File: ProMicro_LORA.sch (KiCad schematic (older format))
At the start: 44 parts, among them J1 SMA, J2 COAX, U1 SX1276, U2 AS179-92LF, Y1 32Mhz

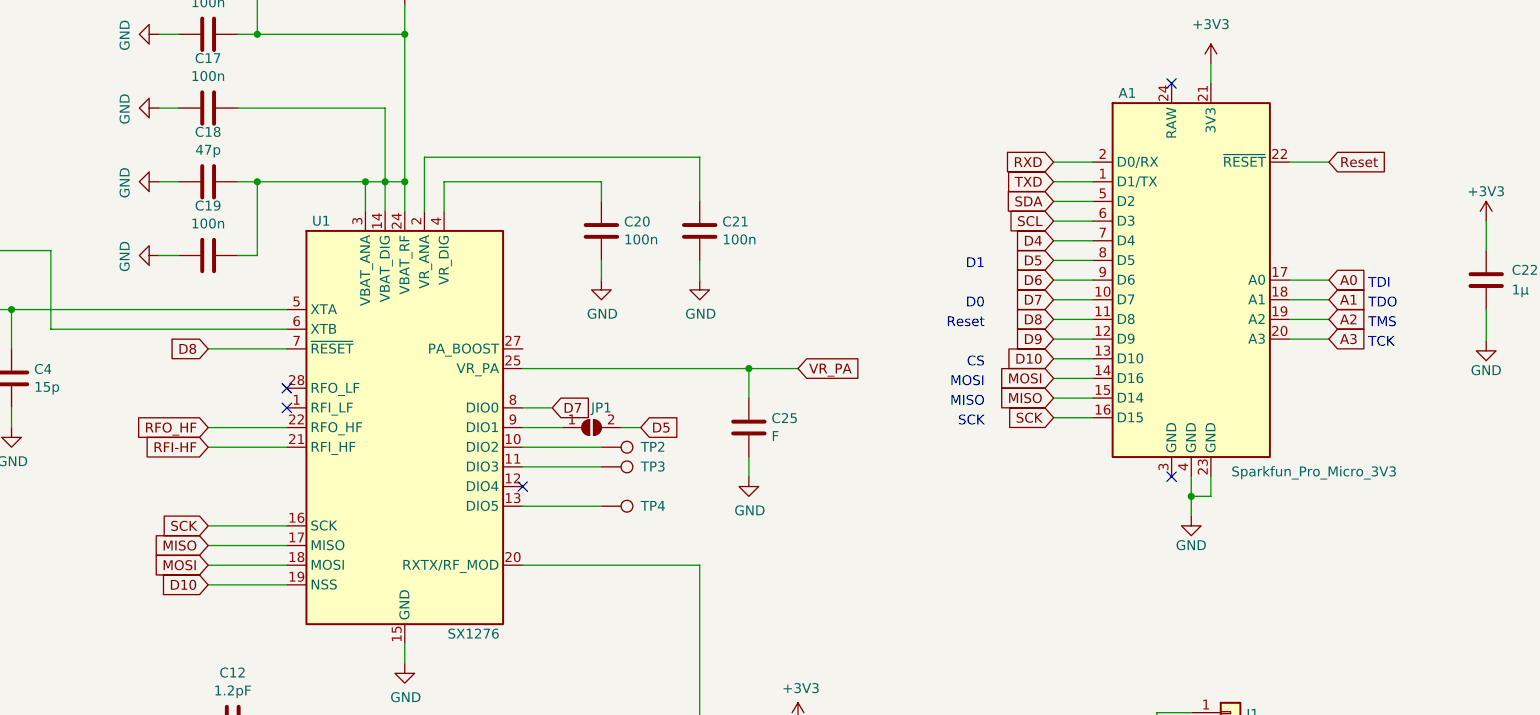
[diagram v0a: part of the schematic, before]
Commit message: kicad-exports
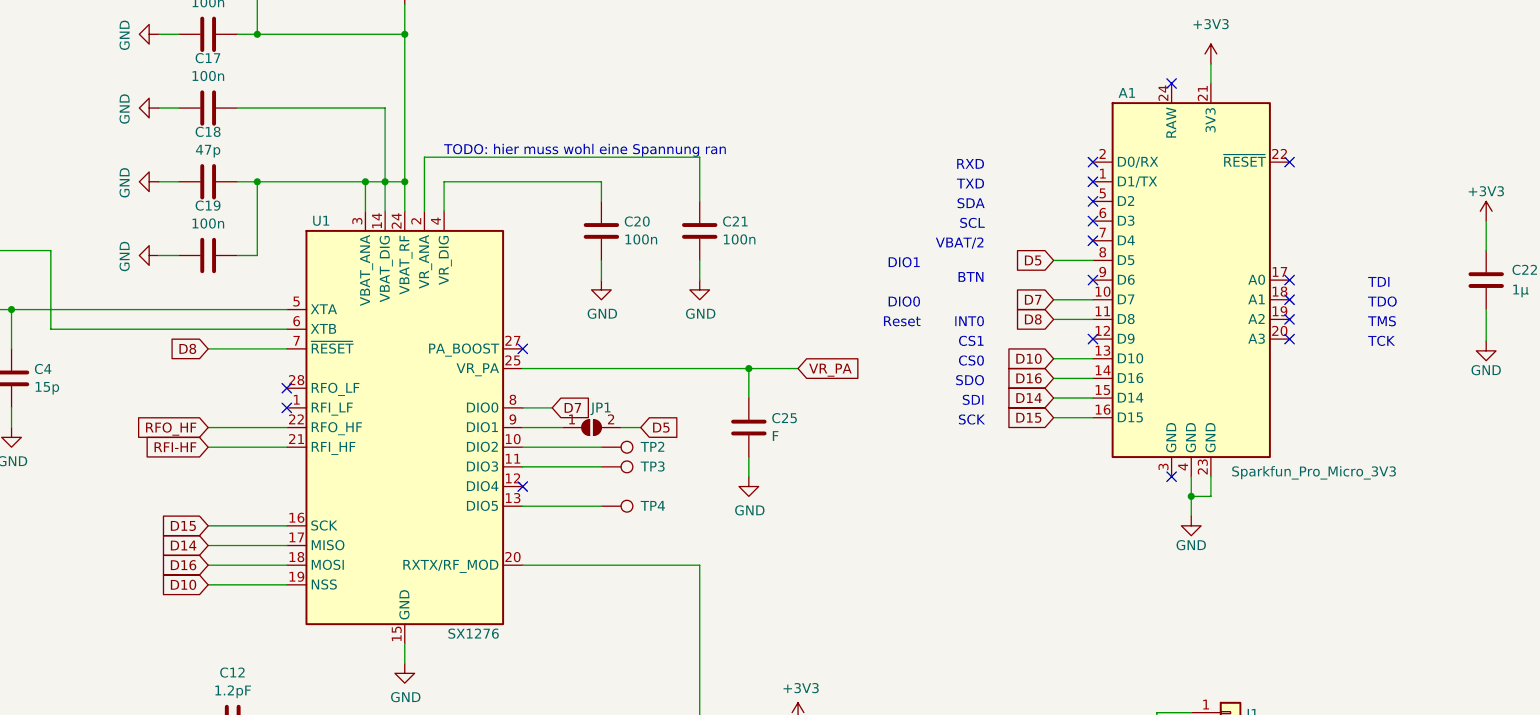
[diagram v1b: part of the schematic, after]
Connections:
- net A0: no longer names the net of A1.17 (A0)
- net A1: no longer names the net of A1.18 (A1)
- net A2: no longer names the net of A1.19 (A2)
- net A3: no longer names the net of A1.20 (A3)
- net D4: no longer names the net of A1.7 (D4)
- net D6: no longer names the net of A1.9 (D6)
- net D9: no longer names the net of A1.12 (D9)
- net MISO renamed D14
- net MOSI renamed D16
- net RXD: no longer names the net of A1.2 (D0/RX)
- net Reset: no longer names the net of A1.22 (~RESET)
- net SCK renamed D15
- net SCL: no longer names the net of A1.6 (D3)
- net SDA: no longer names the net of A1.5 (D2)
- net TXD: no longer names the net of A1.1 (D1/TX)
- no-connect marks 5 -> 18
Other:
- note added: "BTN"
- note added: "CS0"
- note added: "CS1"
- note added: "DIO0"
- note added: "DIO1"
- note added: "INT0"
- note added: "RXD"
- note added: "SCL"
- note added: "SDA"
- note added: "SDI"
- note added: "SDO"
- note added: "TODO: hier muss wohl eine Spannung ran"
- note added: "TXD"
- note added: "VBAT/2"
- note removed: "CS"
- note removed: "D0"
- note removed: "D1"
- note removed: "MISO"
- note removed: "MOSI"
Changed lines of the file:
@@
 	4600 3250 4800 3250
 Wire Wire Line
-	7300 1900 7500 1900
-Wire Wire Line
-	7300 2000 7500 2000
-Wire Wire Line
-	7300 2100 7500 2100
-Wire Wire Line
-	7300 2200 7500 2200
-Wire Wire Line
-	7300 2300 7500 2300
-Wire Wire Line
 	7300 2400 7500 2400
 Wire Wire Line
-	7300 2500 7500 2500
-Wire Wire Line
 	7300 2600 7500 2600
 Wire Wire Line
 	7300 2700 7500 2700
 Wire Wire Line
-	7300 2800 7500 2800
-Wire Wire Line
 	7300 2900 7500 2900
 Wire Wire Line
@@
 	7300 3200 7500 3200
 Wire Wire Line
-	8500 1900 8700 1900
-Wire Wire Line
-	8500 2500 8700 2500
-Wire Wire Line
-	8500 2600 8700 2600
-Wire Wire Line
-	8500 2700 8700 2700
-Wire Wire Line
-	8500 2800 8700 2800
-Wire Wire Line
 	1475 5150 1250 5150
 Wire Wire Line
@@
 Wire Wire Line
 	4100 1875 5500 1875
-Text Notes 6950 2650 2    50   ~ 0
-D0
-Text Notes 6950 2750 2    50   ~ 0
+Text Notes 6625 2650 2    50   ~ 0
+DIO0
+Text Notes 6625 2750 2    50   ~ 0
 Reset
 Text Notes 6950 2950 2    50   ~ 0
-CS
+CS0
 Text Notes 8900 2550 0    50   ~ 0
 TDI
@@
 RFI-HF
 Text GLabel 3000 3750 0    50   Input ~ 0
-SCK
-Text GLabel 3000 3850 0    50   Input ~ 0
-MISO
-Text GLabel 3000 3950 0    50   Input ~ 0
-MOSI
+D15
 Text GLabel 3000 4050 0    50   Input ~ 0
 D10
@@
 Text GLabel 6000 2950 2    50   Input ~ 0
 VR_PA
-Text GLabel 7300 1900 0    50   Input ~ 0
-RXD
-Text GLabel 7300 2000 0    50   Input ~ 0
-TXD
-Text GLabel 7300 2100 0    50   Input ~ 0
-SDA
-Text GLabel 7300 2200 0    50   Input ~ 0
-SCL
-Text GLabel 7300 2300 0    50   Input ~ 0
-D4
 Text GLabel 7300 2400 0    50   Input ~ 0
 D5
-Text GLabel 7300 2500 0    50   Input ~ 0
-D6
 Text GLabel 7300 2600 0    50   Input ~ 0
 D7
 Text GLabel 7300 2700 0    50   Input ~ 0
 D8
-Text GLabel 7300 2800 0    50   Input ~ 0
-D9
 Text GLabel 7300 2900 0    50   Input ~ 0
 D10
 Text GLabel 7300 3000 0    50   Input ~ 0
-MOSI
+D16
 Text GLabel 7300 3100 0    50   Input ~ 0
-MISO
+D14
 Text GLabel 7300 3200 0    50   Input ~ 0
-SCK
-Text GLabel 8700 1900 2    50   Input ~ 0
-Reset
-Text GLabel 8700 2500 2    50   Input ~ 0
-A0
-Text GLabel 8700 2600 2    50   Input ~ 0
-A1
-Text GLabel 8700 2700 2    50   Input ~ 0
-A2
-Text GLabel 8700 2800 2    50   Input ~ 0
-A3
+D15
 $Comp
 L Connector:TestPoint TP2
@@
 	6500 5250 6500 5600
 Text Notes 6950 3050 2    50   ~ 0
-MOSI
+SDO
 Text Notes 6950 3150 2    50   ~ 0
-MISO
+SDI
 Text Notes 6950 3250 2    50   ~ 0
 SCK
-Text Notes 6950 2450 2    50   ~ 0
-D1
 NoConn ~ 7900 1500
 $Comp
@@
 	1    0    0    -1
 $EndComp
+Text Notes 6625 2450 2    50   ~ 0
+DIO1
+Text Notes 6950 1950 2    50   ~ 0
+RXD
+Text Notes 6950 2050 2    50   ~ 0
+TXD
+Text Notes 6950 2150 2    50   ~ 0
+SDA
+Text Notes 6950 2250 2    50   ~ 0
+SCL
+Text Notes 6950 2350 2    50   ~ 0
+VBAT/2
+Text Notes 6950 2525 2    50   ~ 0
+BTN
+Text Notes 6950 2850 2    50   ~ 0
+CS1
+Text GLabel 3000 3950 0    50   Input ~ 0
+D16
+Text GLabel 3000 3850 0    50   Input ~ 0
+D14
+Text Notes 6950 2750 2    50   ~ 0
+INT0
+NoConn ~ 8500 2800
+NoConn ~ 8500 2700
+NoConn ~ 8500 2600
+NoConn ~ 8500 2500
+NoConn ~ 7500 2200
+NoConn ~ 7500 2100
+NoConn ~ 7500 2000
+NoConn ~ 7500 1900
+NoConn ~ 7500 2500
+NoConn ~ 7500 2300
+NoConn ~ 8500 1900
+NoConn ~ 4600 2850
+NoConn ~ 7500 2800
+Text Notes 4200 1875 0    50   ~ 0
+TODO: hier muss wohl eine Spannung ran
 $EndSCHEMATC
